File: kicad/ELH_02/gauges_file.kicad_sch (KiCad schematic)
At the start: 28 parts, among them J2 Screw_Terminal_01x03, J3 Screw_Terminal_01x03, J4 Screw_Terminal_01x03, J5 Screw_Terminal_01x03, J6 Screw_Terminal_01x03, J7 Screw_Terminal_01x03, J8 Screw_Terminal_01x03, U14 HX711, U15 HX711, U16 HX711, U17 HX711, U18 HX711, U19 HX711, U2 HX711

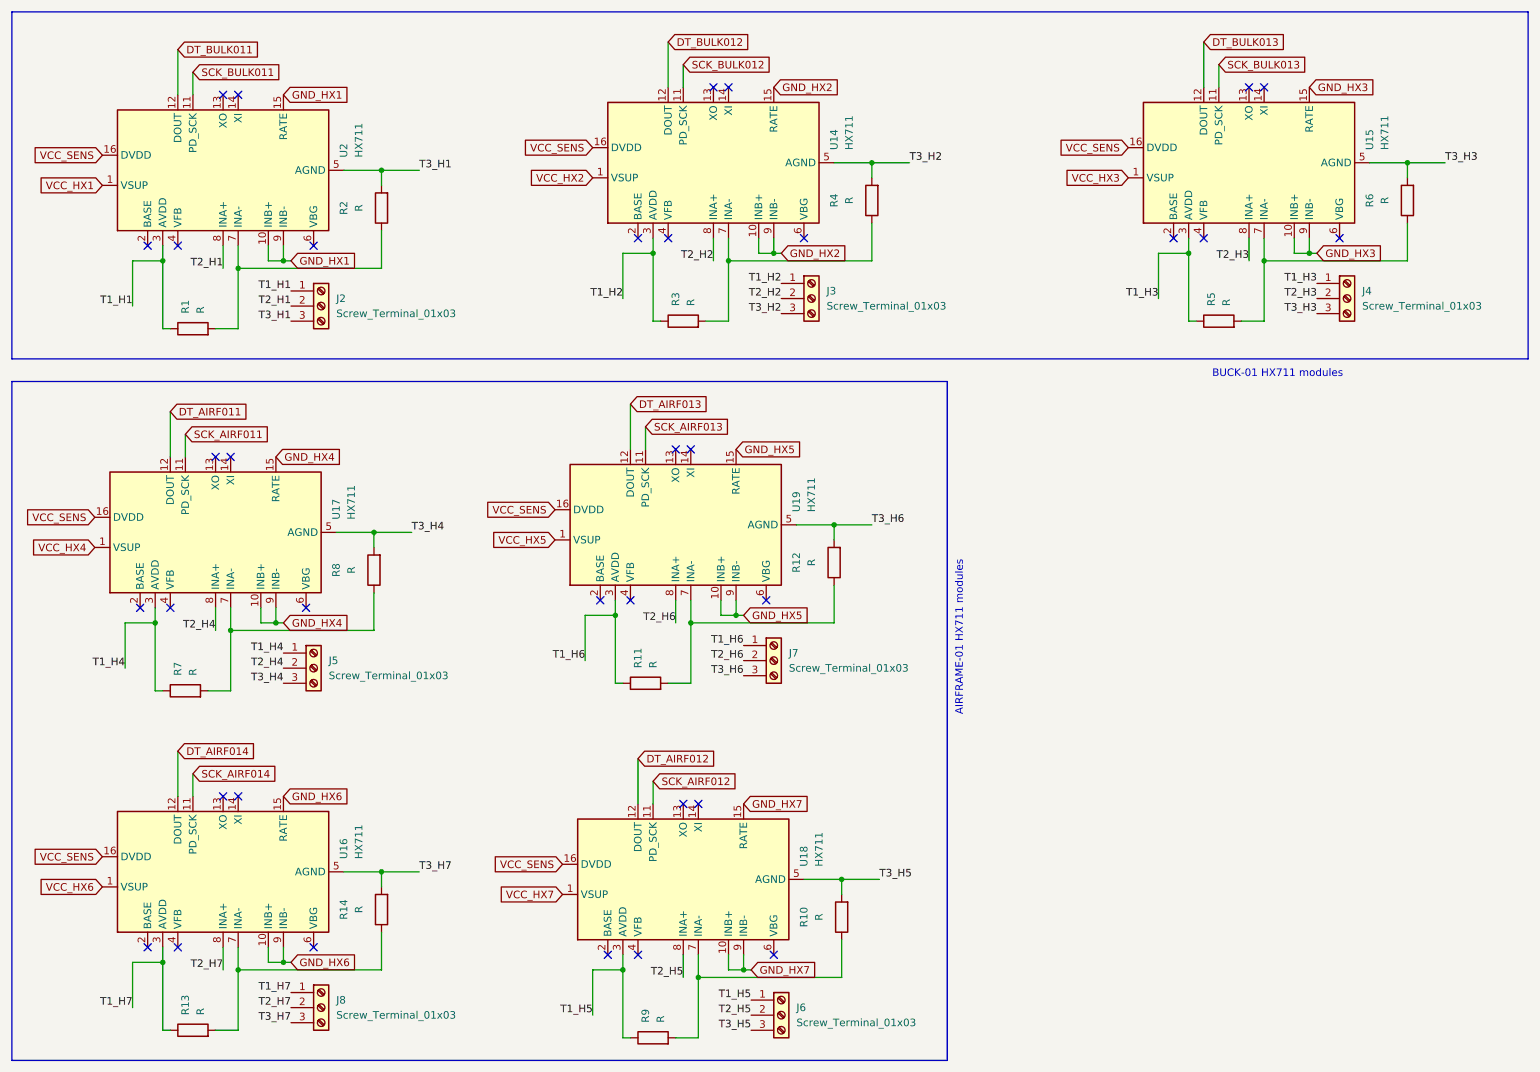
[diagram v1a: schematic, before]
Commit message: Preliminary solution to requested changes
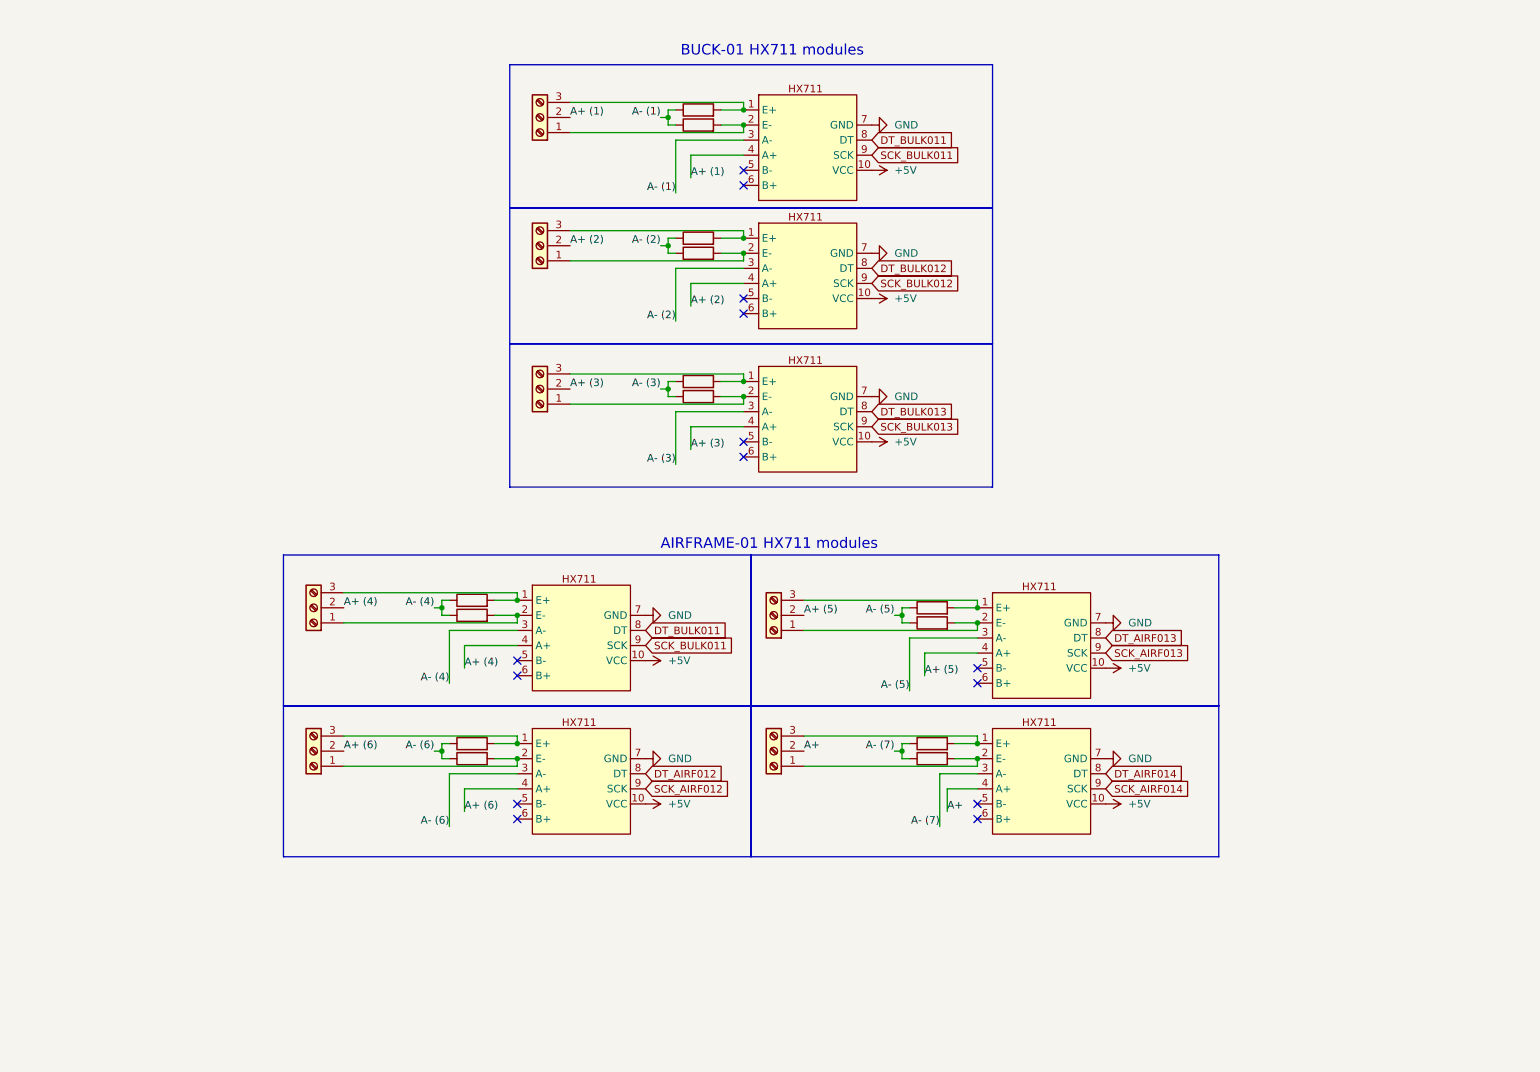
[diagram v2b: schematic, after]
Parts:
- removed J2, J3, J4, J5, J6, J7, J8: Screw_Terminal_01x03, symbol Connector:Screw_Terminal_01x03
- removed R1, R10, R11, R12, R13, R14, R2, R3, R4, R5, R6, R7, R8, R9: R, symbol Device:R
- removed U14, U15, U16, U17, U18, U19, U2: HX711, Package_SO:SOIC-16_3.9x9.9mm_P1.27mm, symbol Analog_ADC:HX711
- added HX711 (x7): Amplifier, symbol C_sym:HX711
- added Resistor (x14): Resistor, symbol Device:R
- added Screw_Terminal_01x03 (x7): Screw Terminal, symbol Connector:Screw_Terminal_01x03
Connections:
- net DT_AIRF012: now also HX711.8 (DT)
- net DT_AIRF013: now also HX711.8 (DT)
- net DT_AIRF014: now also HX711.8 (DT)
- net DT_BULK011: now also HX711.8 (DT), HX711.8 (DT)
- net DT_BULK012: now also HX711.8 (DT)
- net DT_BULK013: now also HX711.8 (DT)
- net SCK_AIRF012: now also HX711.9 (SCK)
- net SCK_AIRF013: now also HX711.9 (SCK)
- net SCK_AIRF014: now also HX711.9 (SCK)
- net SCK_BULK011: now also HX711.9 (SCK), HX711.9 (SCK)
- net SCK_BULK012: now also HX711.9 (SCK)
- net SCK_BULK013: now also HX711.9 (SCK)
- new net: HX711.2 (E-), Resistor.2, Screw_Terminal_01x03.1 (Pin_1) (x7)
- new net: HX711.1 (E+), Resistor.2, Screw_Terminal_01x03.3 (Pin_3) (x7)
- new net +5V: HX711.10 (VCC), HX711.10 (VCC), HX711.10 (VCC), HX711.10 (VCC), HX711.10 (VCC), HX711.10 (VCC), HX711.10 (VCC)
- new net A+: HX711.4 (A+), Screw_Terminal_01x03.2 (Pin_2)
- new net A+ (1): HX711.4 (A+), Screw_Terminal_01x03.2 (Pin_2)
- new net A+ (2): HX711.4 (A+), Screw_Terminal_01x03.2 (Pin_2)
- new net A+ (3): HX711.4 (A+), Screw_Terminal_01x03.2 (Pin_2)
- new net A+ (4): HX711.4 (A+), Screw_Terminal_01x03.2 (Pin_2)
- new net A+ (5): HX711.4 (A+), Screw_Terminal_01x03.2 (Pin_2)
- new net A+ (6): HX711.4 (A+), Screw_Terminal_01x03.2 (Pin_2)
- new net A- (1): HX711.3 (A-), Resistor.1, Resistor.1
- new net A- (2): HX711.3 (A-), Resistor.1, Resistor.1
- new net A- (3): HX711.3 (A-), Resistor.1, Resistor.1
- new net A- (4): HX711.3 (A-), Resistor.1, Resistor.1
- new net A- (5): HX711.3 (A-), Resistor.1, Resistor.1
- new net A- (6): HX711.3 (A-), Resistor.1, Resistor.1
- new net A- (7): HX711.3 (A-), Resistor.1, Resistor.1
- new net GND: HX711.7 (GND), HX711.7 (GND), HX711.7 (GND), HX711.7 (GND), HX711.7 (GND), HX711.7 (GND), HX711.7 (GND)
- no-connect marks 35 -> 14
